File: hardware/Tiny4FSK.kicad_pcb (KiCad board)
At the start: 4 copper layers, 20 x 71 mm, 89 parts, among them J10 GPIO_ROW, J2 PWR, J5 USB Breakout, J7 GCT-4105, J8 SWD, J9 Counterpoise, SW1 PWR, SW2 RST, U1 BME280, U10 USBLC6-2SC6, U11 ATGM336H, U3 TPS61200DRC, U5 ATSAMD21G18A-A, U6 Si4463, U7 XC6210B332MR, U9 TPS2116DRL

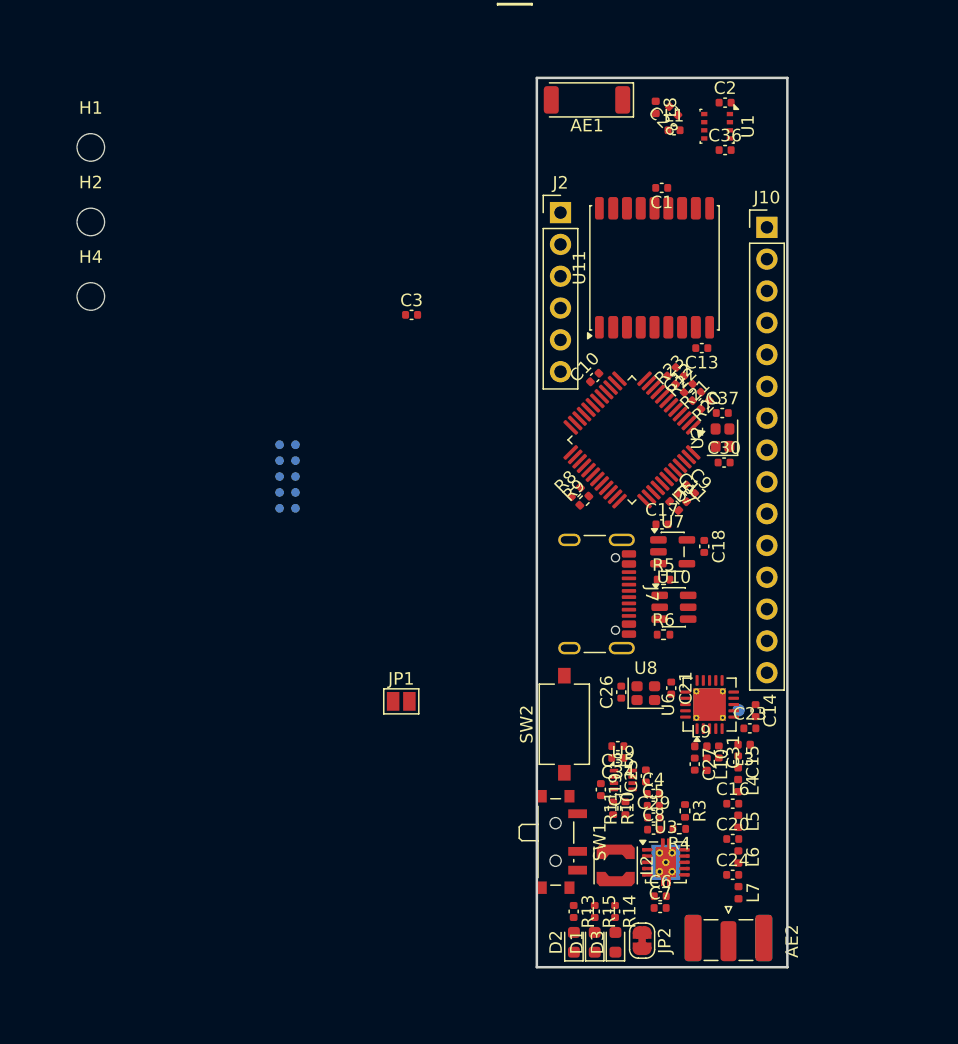
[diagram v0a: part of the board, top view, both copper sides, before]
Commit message: draft of final layout
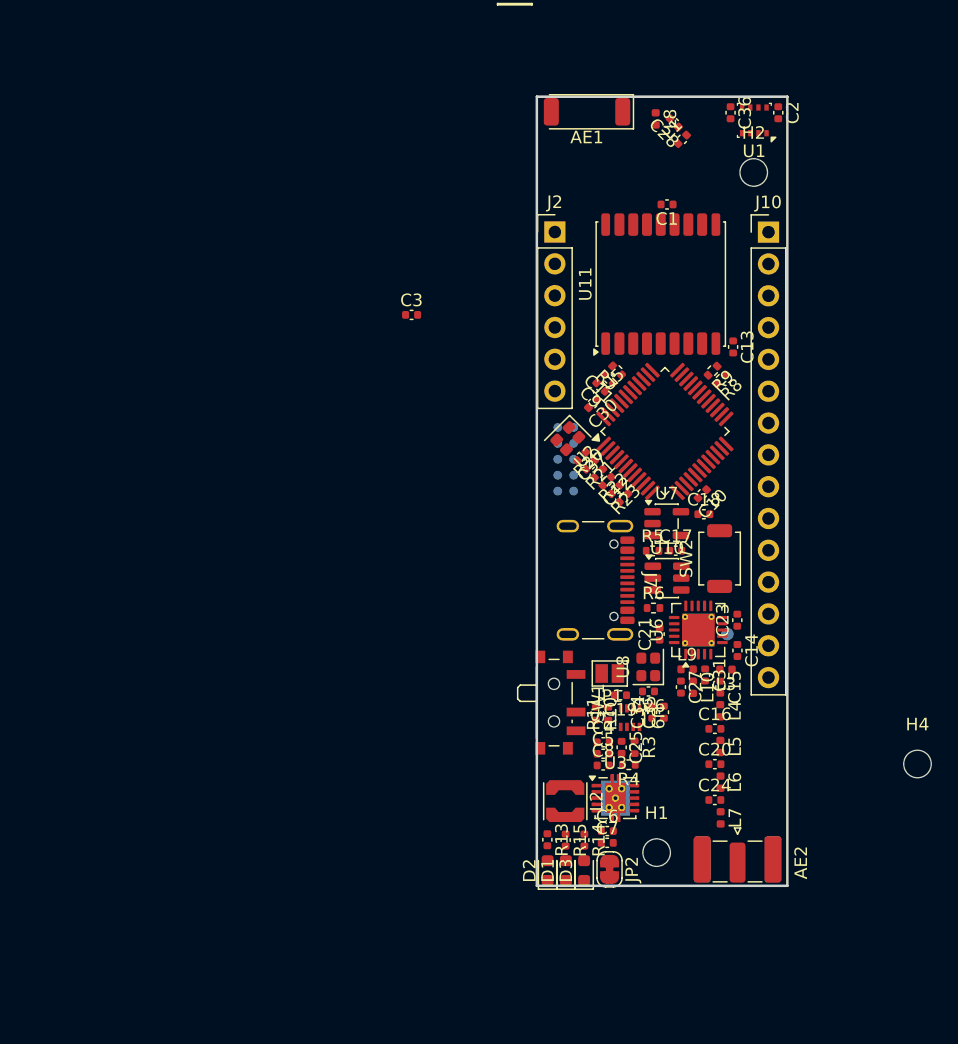
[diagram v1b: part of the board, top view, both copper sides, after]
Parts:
- removed C29: 100nF, Capacitor_SMD:C_0402_1005Metric
- SW2: footprint Button_Switch_SMD:SW_Tactile_SPST_NO_Straight_CK_PTS636Sx25SMTRLFS -> Button_Switch_SMD:SW_SPST_TS-1088-xR020
- moved H4 75.8 mm to (158.6, 114.2)
- moved H1 72.2 mm to (137.7, 121.3)
- moved H2 53.1 mm to (145.5, 67.0)
- moved J8 22.3 mm to (130.5, 89.9), turned to 0 degrees
- moved SW2 18.1 mm to (142.8, 97.8)
- moved JP1 16.8 mm to (134.0, 107.0), turned to 180 degrees
- moved R8 14.7 mm to (142.9, 83.5), turned to -135 degrees
- moved R9 14.6 mm to (142.2, 82.8), turned to -135 degrees
- moved C10 12.7 mm to (141.4, 92.6), turned to -135 degrees
- moved U2 12.4 mm to (130.6, 88.2), turned to -135 degrees
- moved C37 11.8 mm to (131.7, 89.6), turned to -135 degrees
- moved R7 11.7 mm to (134.6, 82.8), turned to 135 degrees
- moved C30 11.5 mm to (132.6, 85.4), turned to -135 degrees
- moved C11 11.1 mm to (133.9, 83.5), turned to 135 degrees
- moved SW1 11.1 mm to (129.9, 109.3)
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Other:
- board size 20 x 71 mm -> 20 x 63 mm
